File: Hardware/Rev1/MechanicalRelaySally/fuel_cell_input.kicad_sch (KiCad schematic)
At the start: 9 parts, among them J2 VP0265540000G, Q1 NMOS, Q2 NMOS, U1 ACS72981LLRATR-050B3, U2 LM74700

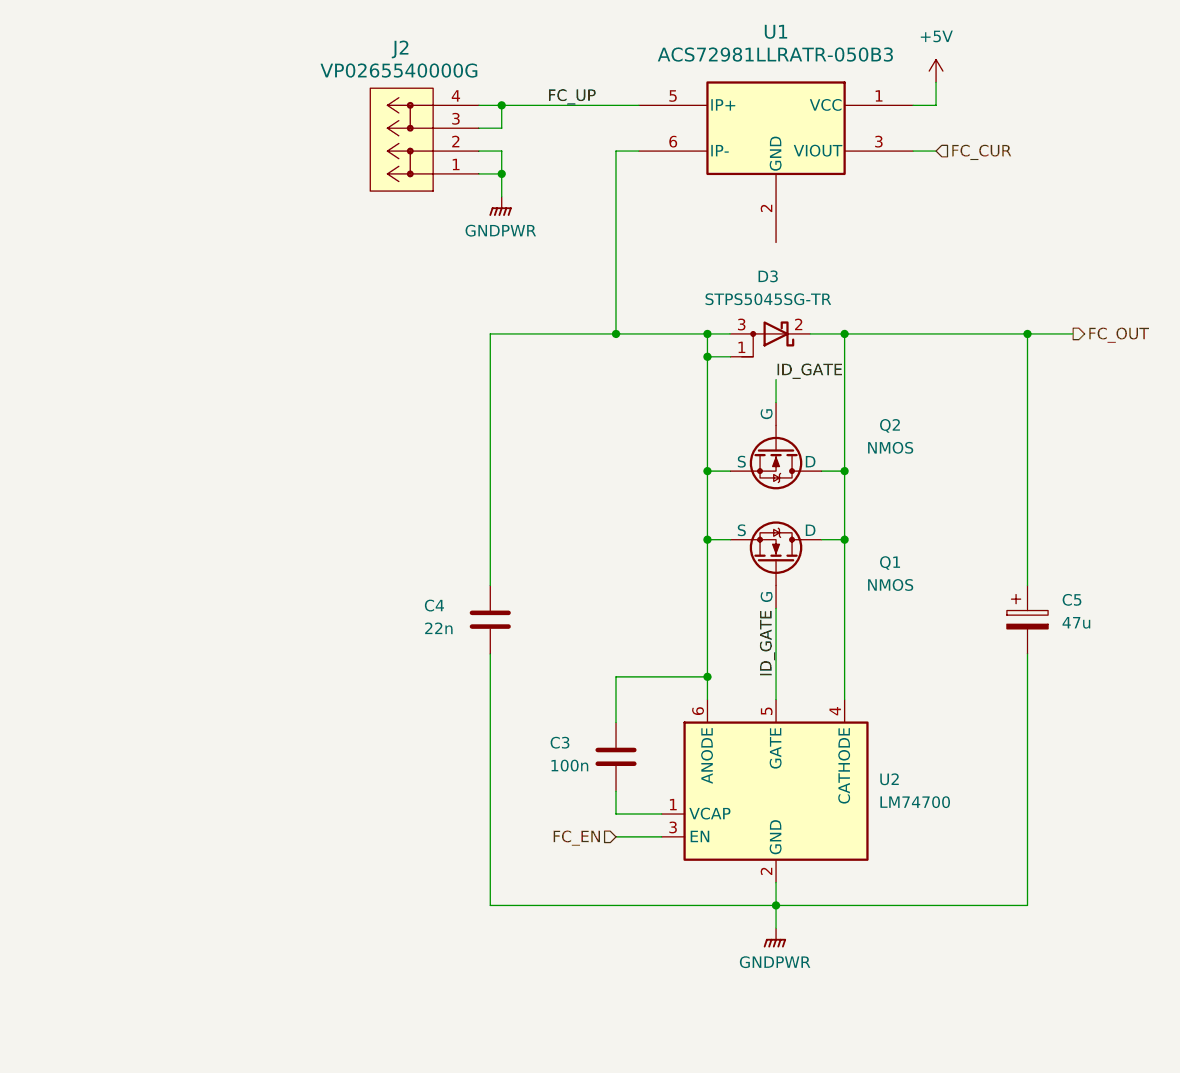
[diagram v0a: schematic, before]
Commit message: A
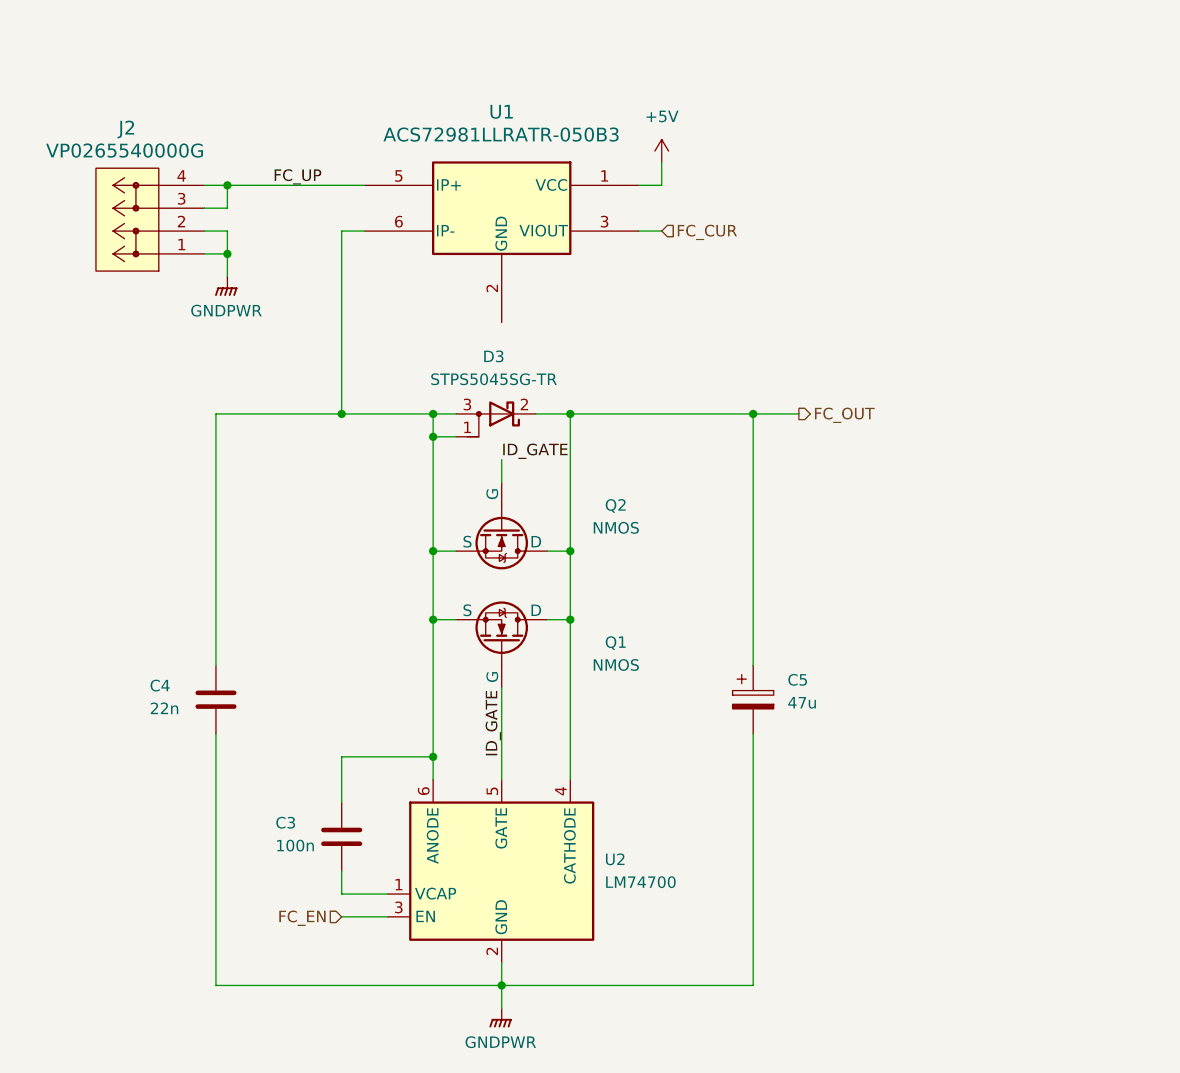
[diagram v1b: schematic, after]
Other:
- moved on the sheet: C3, C4, C5, D3, J2, Q1, Q2, U1, U2
